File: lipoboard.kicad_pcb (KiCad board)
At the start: 2 copper layers, 54.5 x 35 mm, 50 parts, among them J1 USB_C_Receptacle_PowerOnly_24P, SW1 SW_DIP_x01, U1 TPS2116DRL, U3 DW01A, U5 TPS63001

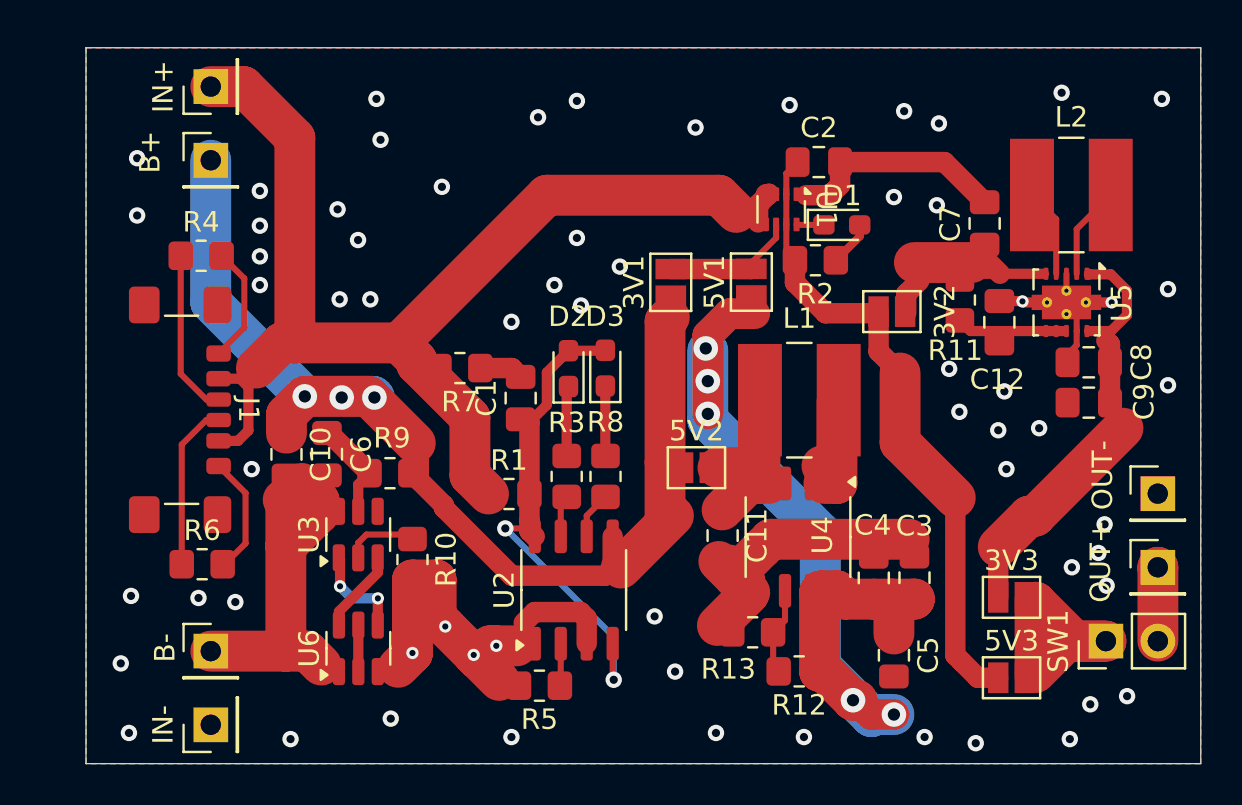
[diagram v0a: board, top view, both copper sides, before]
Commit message: Init!
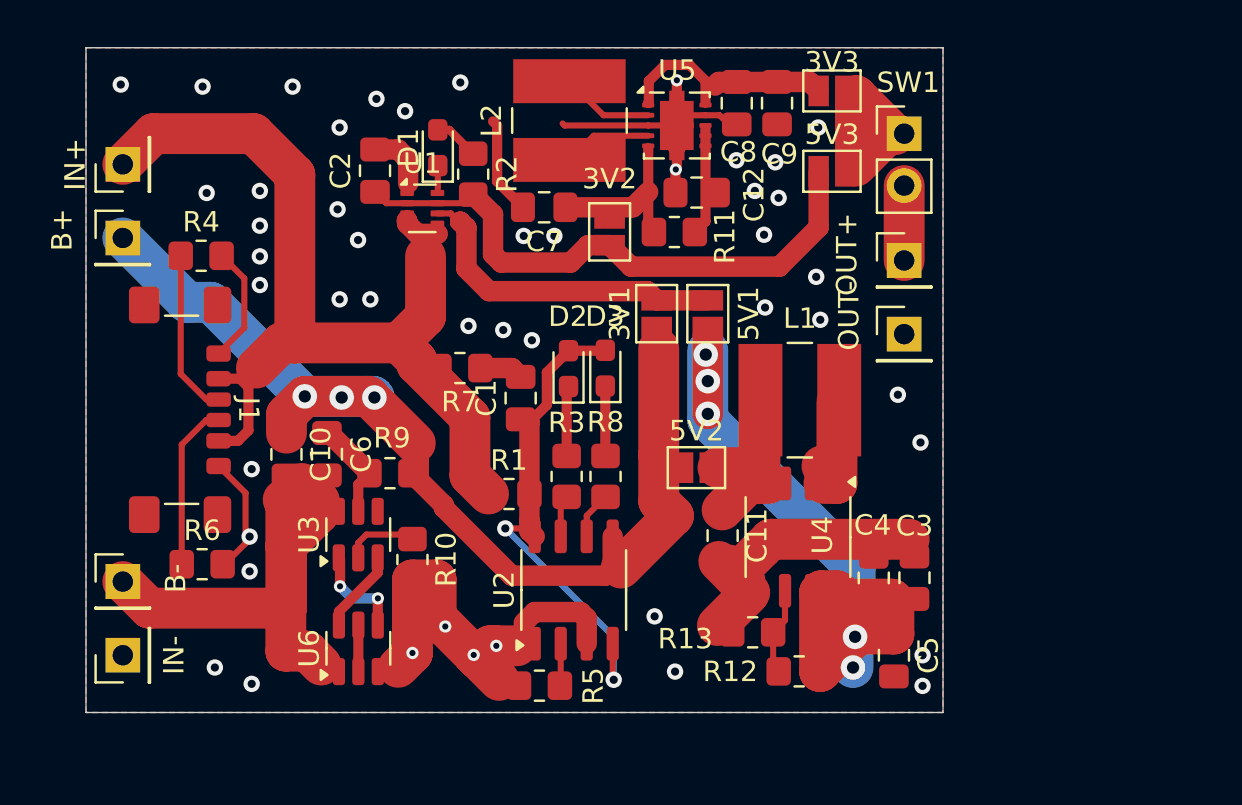
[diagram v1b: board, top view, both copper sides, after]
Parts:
- moved SW1 26.7 mm to (99.4, 113.7), turned to 0 degrees
- moved 3V3 26.3 mm to (95.9, 111.6)
- moved 5V3 26.3 mm to (95.9, 115.5)
- moved L2 24.8 mm to (83.0, 113.1), turned to -90 degrees
- moved C2 21.7 mm to (73.5, 115.5), turned to 90 degrees
- moved C7 21.5 mm to (81.8, 117.3), turned to 180 degrees
- moved C8 21.4 mm to (91.2, 112.2), turned to -90 degrees
- moved C9 21.1 mm to (93.2, 112.2), turned to -90 degrees
- moved U5 20.9 mm to (88.3, 113.3), turned to 0 degrees
- moved D1 20.1 mm to (76.6, 114.4), turned to 90 degrees
- moved OUT+ 19.5 mm to (99.4, 119.9)
- moved U1 17.6 mm to (75.8, 117.3), turned to 0 degrees
- moved R2 17.3 mm to (78.3, 115.7), turned to -90 degrees
- moved C12 16.1 mm to (89.3, 116.6), turned to 180 degrees
- moved OUT- 14.6 mm to (99.4, 123.5)
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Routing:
- net VBUS: track 58.9 -> 46.8 mm
- net Net-(3V1-B): track 6.62 -> 16.1 mm
- net 3.3VOUT: track 19.7 -> 10.9 mm
- net Net-(B-1-Pin_1): track 17.2 -> 25.1 mm
- net 5VOUT: track 43.9 -> 38.1 mm
- net Net-(3V3-B): track 14.1 -> 10.6 mm
- net Net-(3V2-A): track 11.9 -> 8.58 mm
- net MUXOUT: track 31.9 -> 28.9 mm
- net VBAT: track 53.7 -> 51.0 mm
- net GND: track 64.8 -> 66.0 mm, vias 64 -> 47
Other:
- board size 54.5 x 35 mm -> 41.9 x 32.5 mm
